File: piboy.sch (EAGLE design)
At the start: 78 parts, among them CN4 MicroUSB, T1 MMUN2133LT1G, U1 TPS61090RSAR, U2 MCP73871

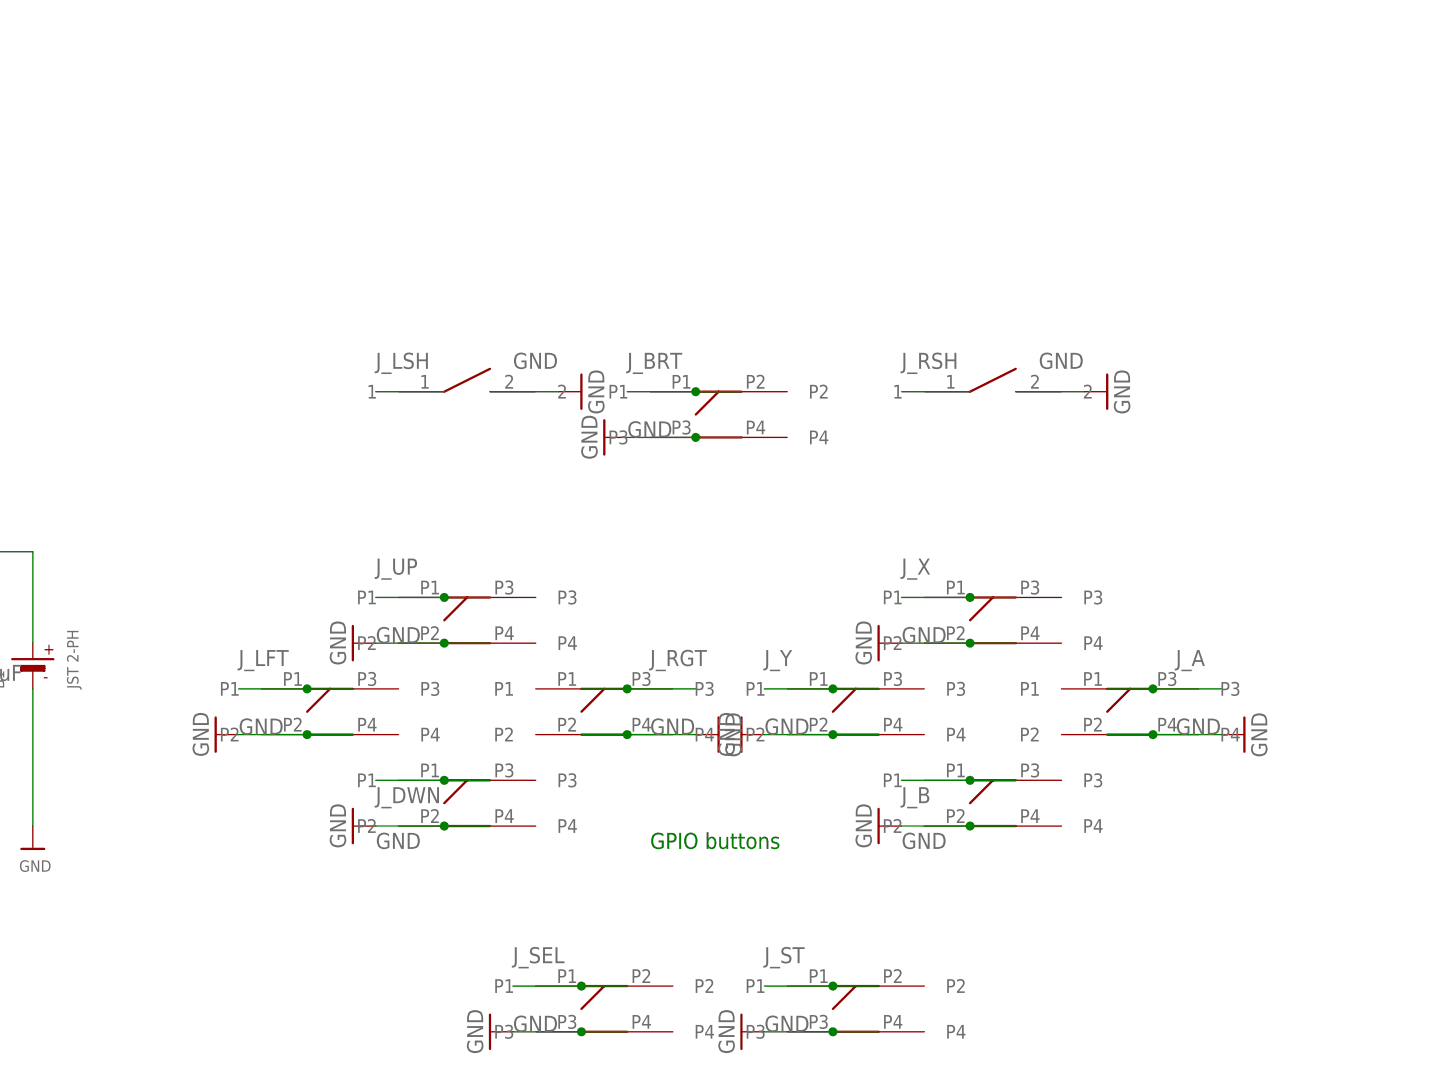
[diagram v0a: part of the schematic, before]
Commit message: -did some wiring
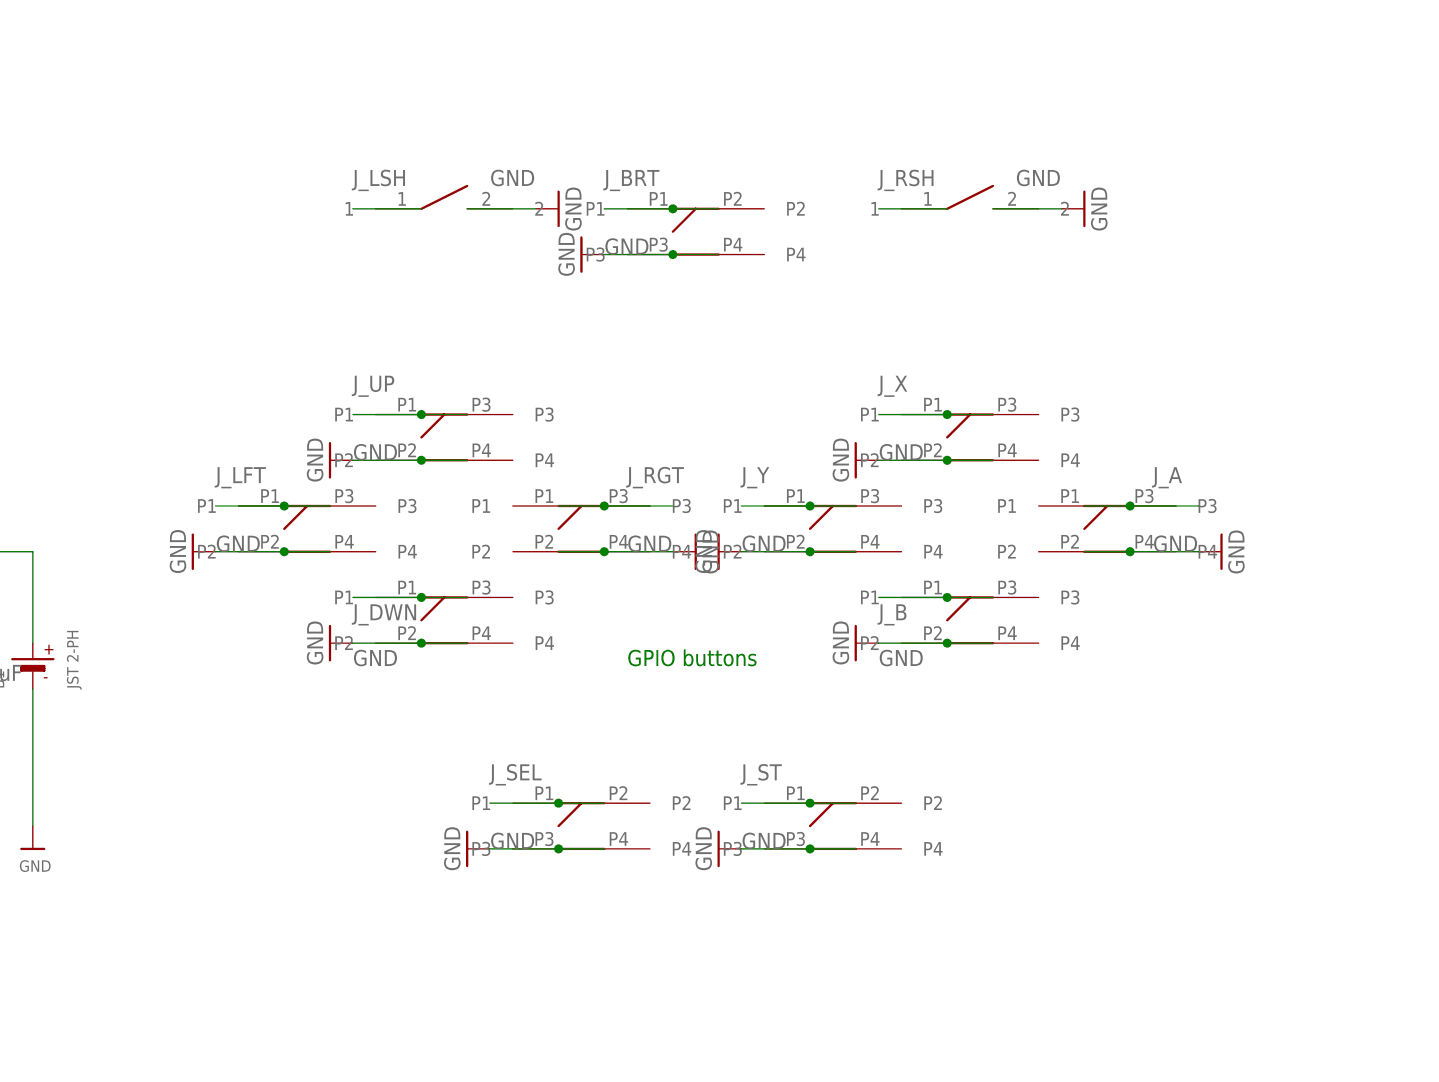
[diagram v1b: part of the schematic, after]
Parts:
- C1, C7: device adafruit:C-USC0805 -> resistor:C-USC1210
- C6: device adafruit:C-USC1210 -> resistor:C-USC1210
